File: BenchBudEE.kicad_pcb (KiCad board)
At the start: 4 copper layers, 165.1 x 63.5 mm, 0 parts

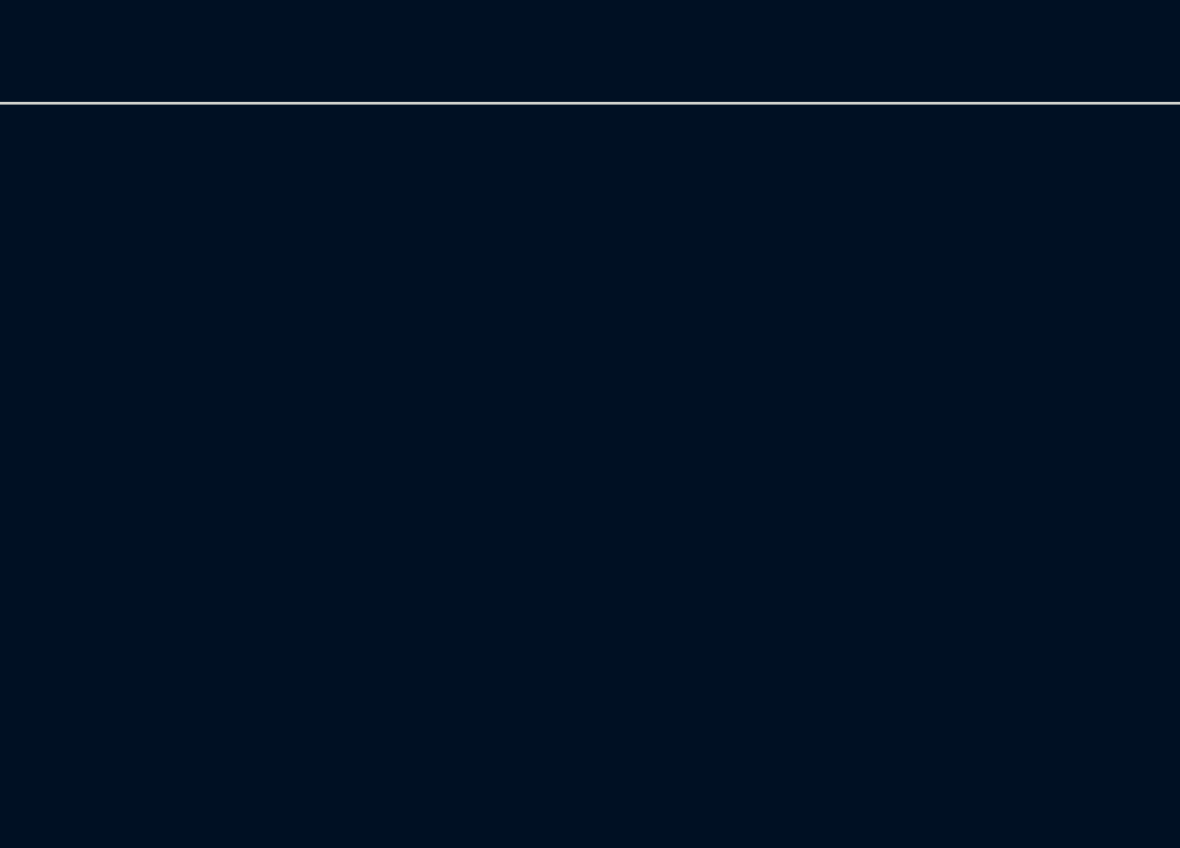
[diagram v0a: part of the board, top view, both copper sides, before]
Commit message: Placed Relay Module Components
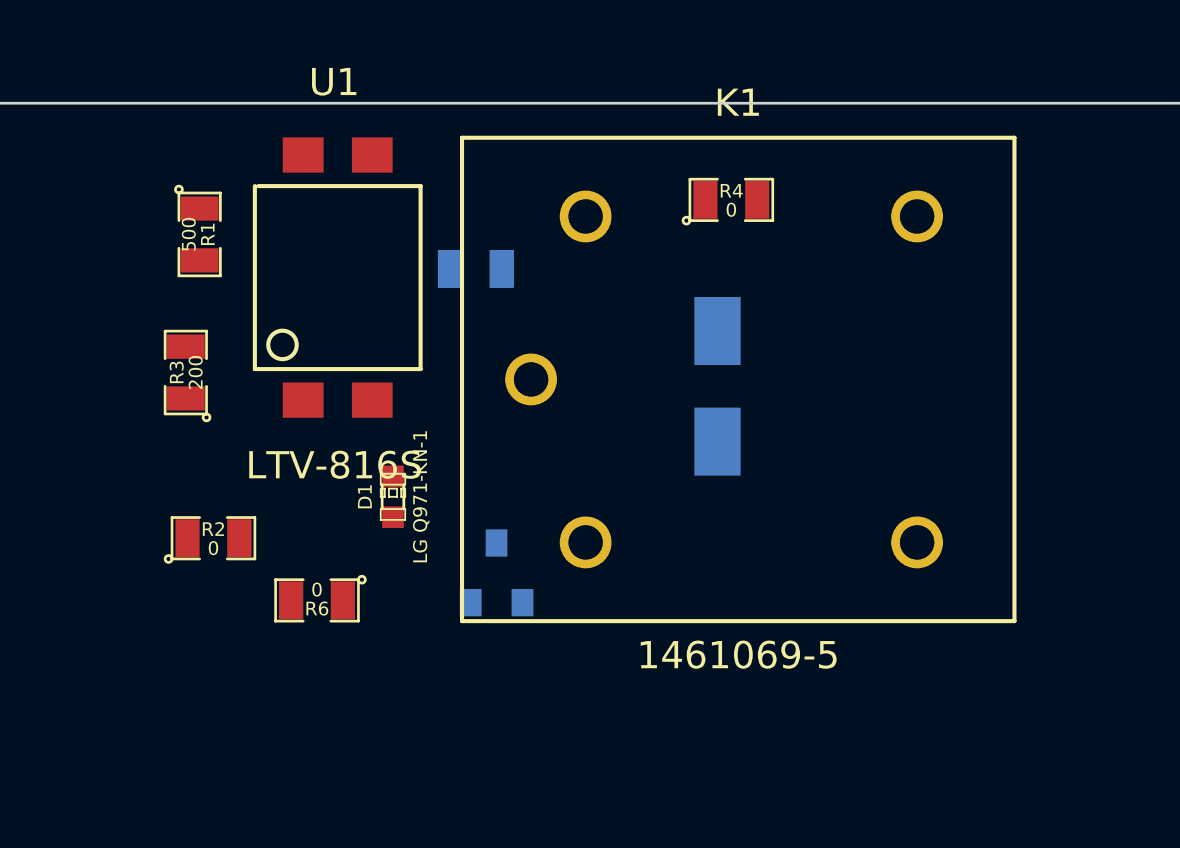
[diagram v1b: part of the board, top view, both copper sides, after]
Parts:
- added D1: LG Q971-KN-1, LEDs:LED-0603, F.Cu at (257.8, 128.8)
- added D2: B130-13-F, BenchBudEE:SMA, B.Cu at (269.7, 126.7)
- added K1: 1461069-5, BenchBudEE:TE-SPDT, F.Cu at (262.9, 124.5)
- added Q1: 2N3904, SMD_Packages:SOT23, B.Cu at (261.6, 131.6)
- added R1: 500, SMD_Packages:SM0805, F.Cu at (250.7, 119.1)
- added R2: 0, SMD_Packages:SM0805, F.Cu at (251.2, 130.3)
- added R3: 200, SMD_Packages:SM0805, F.Cu at (250.2, 124.2)
- added R4: 0, SMD_Packages:SM0805, F.Cu at (270.3, 117.9)
- added R5: 100, SMD_Packages:SM0805, B.Cu at (260.9, 120.4)
- added R6: 0, SMD_Packages:SM0805, F.Cu at (255.0, 132.6)
- added U1: LTV-816S, BenchBudEE:4-SMD, F.Cu at (254.5, 125.2)
